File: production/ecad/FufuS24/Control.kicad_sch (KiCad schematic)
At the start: 28 parts, among them IC1 NLVPCA9535EDTR2G, J2 Conn_01x02, U1 RP2040, U2 W25Q128JVS

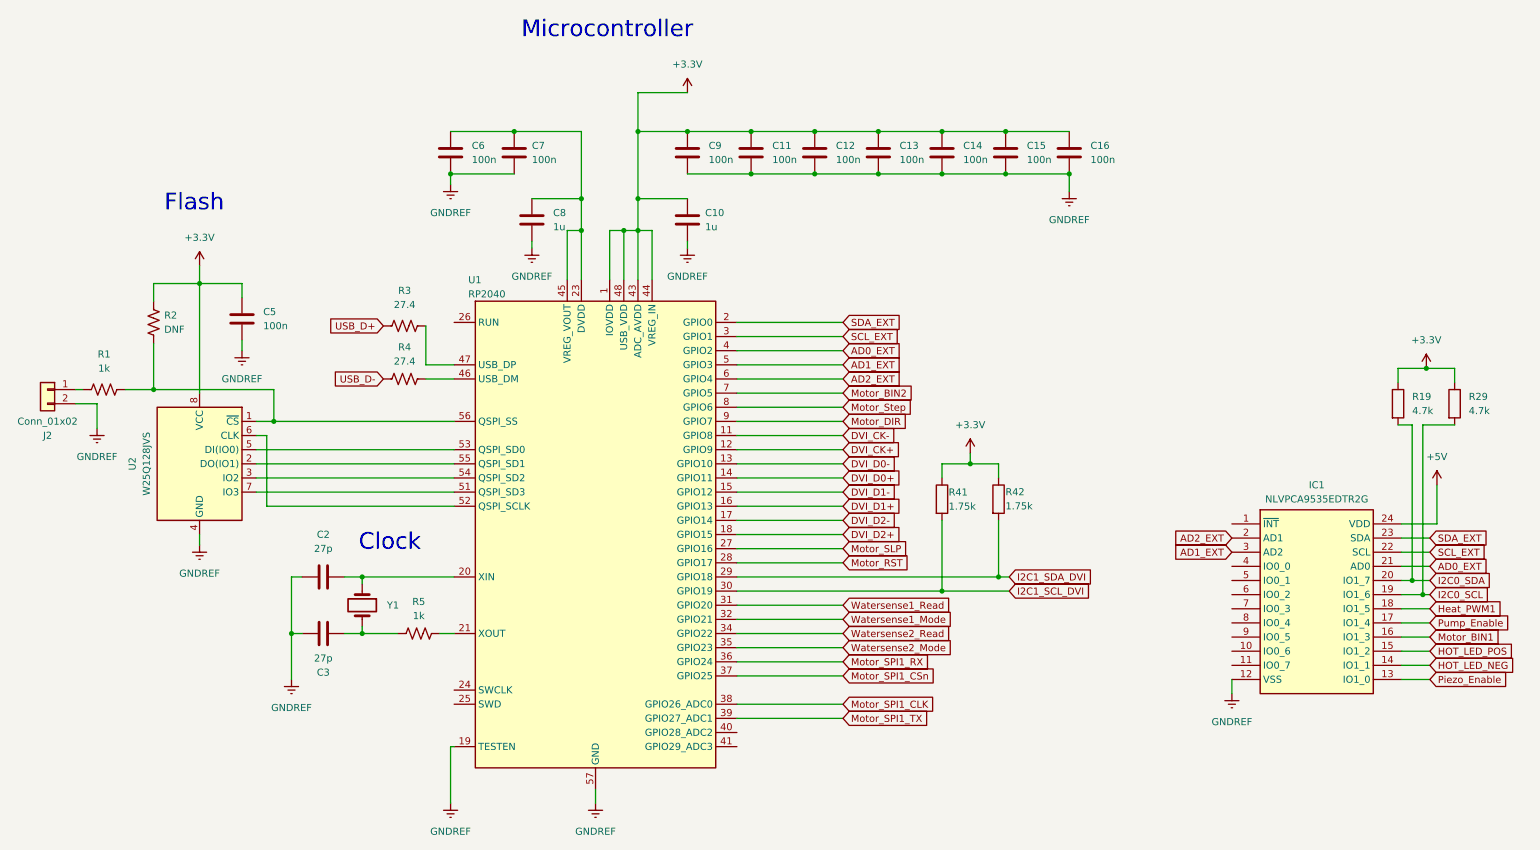
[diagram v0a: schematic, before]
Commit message: Made GPIO changes
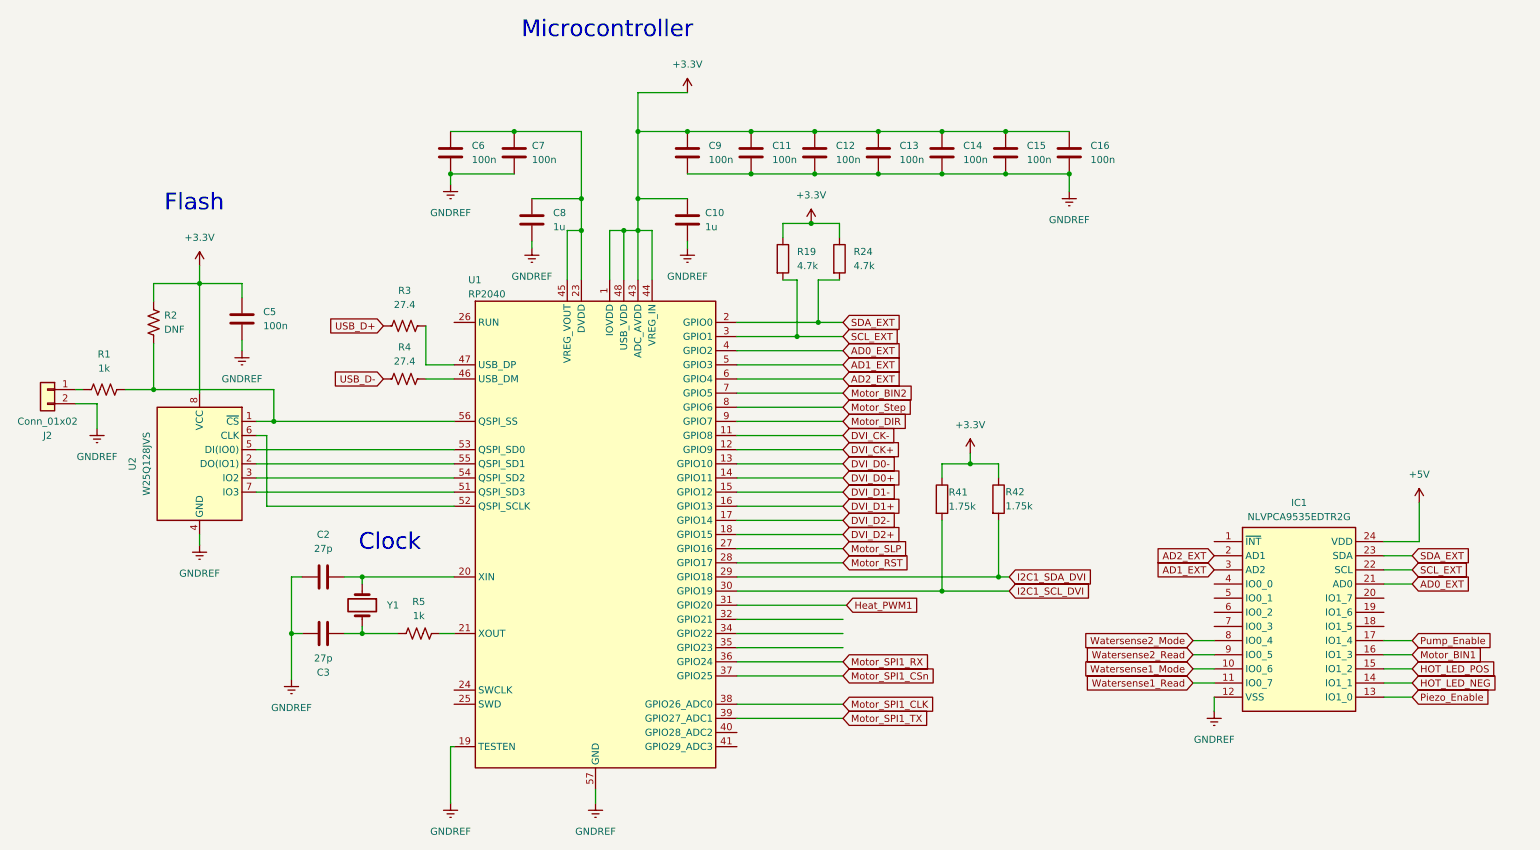
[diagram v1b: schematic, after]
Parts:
- removed R29: 4.7k, footprints:RESC2012X60N, symbol Device:R
- added R24: 4.7k, footprints:RESC2012X60N, symbol Device:R
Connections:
- net +3.3V: now also R24.1
- net Heat_PWM1: now also U1.31 (GPIO20); no longer IC1.18 (IO1_5)
- net SCL_EXT: now also R19.2
- net SDA_EXT: now also R24.2
- net Watersense1_Mode: now also IC1.10 (IO0_6); no longer U1.32 (GPIO21)
- net Watersense1_Read: now also IC1.11 (IO0_7); no longer U1.31 (GPIO20)
- net Watersense2_Mode: now also IC1.8 (IO0_4); no longer U1.35 (GPIO23)
- net Watersense2_Read: now also IC1.9 (IO0_5); no longer U1.34 (GPIO22)
- net I2C0_SCL: no longer names the net of IC1.19 (IO1_6)
- net I2C0_SDA: no longer names the net of IC1.20 (IO1_7)
- net I2C0_SDA: no longer R19.2
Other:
- moved on the sheet: IC1

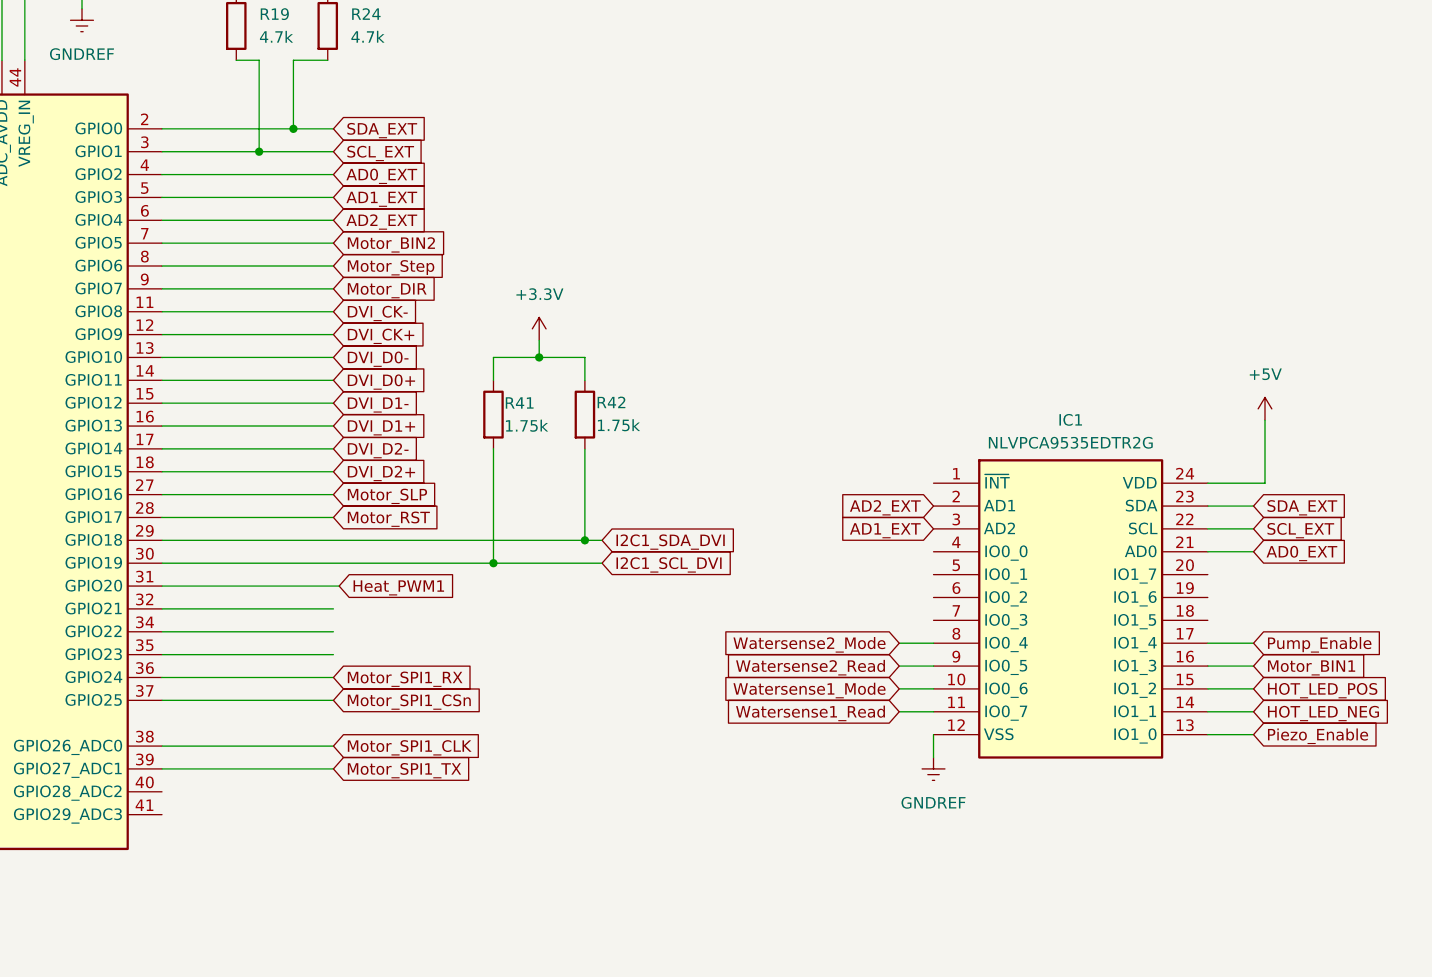
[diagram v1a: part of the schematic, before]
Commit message: Big layout push
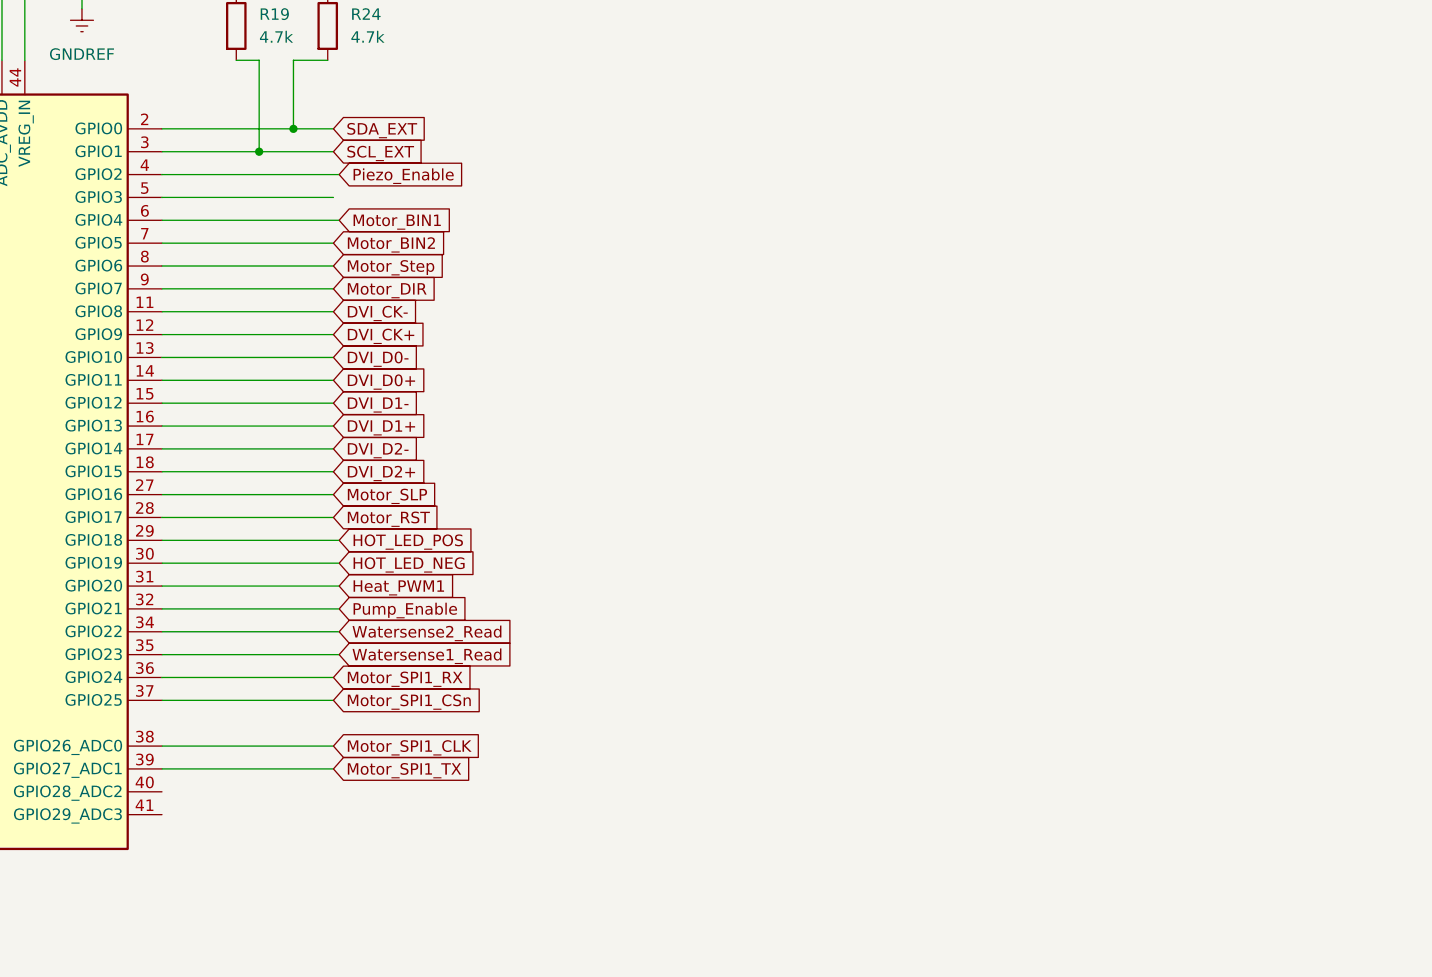
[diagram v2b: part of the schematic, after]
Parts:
- removed IC1: NLVPCA9535EDTR2G, footprints:SOP65P640X120-24N, symbol NLVPCA9535EDTR2G:NLVPCA9535EDTR2G
- removed R41, R42: 1.75k, footprints:RESC2012X60N, symbol Device:R
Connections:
- net AD0_EXT is gone; now on net Piezo_Enable: U1.4 (GPIO2)
- net AD2_EXT is gone; now on net Motor_BIN1: U1.6 (GPIO4)
- net I2C1_SCL_DVI is gone; now on net HOT_LED_NEG: U1.30 (GPIO19)
- net I2C1_SDA_DVI is gone; now on net HOT_LED_POS: U1.29 (GPIO18)
- net Pump_Enable: now also U1.32 (GPIO21)
- net Watersense1_Read: now also U1.35 (GPIO23)
- net Watersense2_Read: now also U1.34 (GPIO22)
- net AD1_EXT: no longer names the net of U1.5 (GPIO3)
